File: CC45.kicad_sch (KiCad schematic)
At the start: 21 parts, among them J1 AVR-ISP-6, SW1 RESET, U1 ATmega32U4-AU, U2 PRTR5V0U2X, X1 XTAL

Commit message: add socket keep out zones
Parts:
- U1: footprint Package_QFP:TQFP-44_10x10mm_P0.8mm -> Package_QFP:TQFP-64_7x7mm_P0.4mm
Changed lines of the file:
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@@
   (junction (at 156.21 165.1) (diameter 0) (color 0 0 0 0))
   (no_connect (at 113.03 170.18))
-  (no_connect (at 64.77 72.39))
-  (no_connect (at 34.29 52.07))
+  (no_connect (at 113.03 154.94))
   (no_connect (at 64.77 36.83))
-  (no_connect (at 113.03 154.94))
   (no_connect (at 64.77 67.31))
   (no_connect (at 64.77 74.93))
+  (no_connect (at 34.29 52.07))
   (no_connect (at 64.77 69.85))
+  (no_connect (at 64.77 72.39))
   (wire (pts (xy 27.94 139.7) (xy 27.94 146.05))
     (stroke (width 0) (type solid) (color 0 0 0 0))
@@
     (property "Reference" "U1" (id 0) (at 39.37 120.65 0))
     (property "Value" "ATmega32U4-AU" (id 1) (at 36.83 123.19 0))
-    (property "Footprint" "Package_QFP:TQFP-44_10x10mm_P0.8mm" (id 2) (at 49.53 74.93 0)
+    (property "Footprint" "Package_QFP:TQFP-64_7x7mm_P0.4mm" (id 2) (at 49.53 74.93 0)
       (effects (font (size 1.27 1.27) italic) hide)
     )

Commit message: switch to 0805
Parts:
- C1, C2, C3, C4, C5, C6, C7, C8: footprint Capacitor_SMD:C_1206_3216Metric_Pad1.42x1.75mm_HandSolder -> Capacitor_SMD:C_0805_2012Metric
- R1, R2, R3, R4, R5, R6: footprint Resistor_SMD:R_1206_3216Metric_Pad1.42x1.75mm_HandSolder -> Resistor_SMD:R_0805_2012Metric
- U1: footprint Package_QFP:TQFP-64_7x7mm_P0.4mm -> libs:QFN44G-0.5-7X7MM
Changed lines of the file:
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@@
       (effects (font (size 1.27 1.27)) (justify right))
     )
-    (property "Footprint" "Resistor_SMD:R_1206_3216Metric_Pad1.42x1.75mm_HandSolder" (id 2) (at 40.64 175.26 0)
+    (property "Footprint" "Resistor_SMD:R_0805_2012Metric" (id 2) (at 40.64 175.26 0)
       (effects (font (size 1.27 1.27)) hide)
     )
@@
     (property "Reference" "R1" (id 0) (at 73.66 85.1916 90))
     (property "Value" "10k" (id 1) (at 73.66 87.503 90))
-    (property "Footprint" "Resistor_SMD:R_1206_3216Metric_Pad1.42x1.75mm_HandSolder" (id 2) (at 73.66 90.17 0)
+    (property "Footprint" "Resistor_SMD:R_0805_2012Metric" (id 2) (at 73.66 90.17 0)
       (effects (font (size 1.27 1.27)) hide)
     )
@@
     (property "Reference" "R5" (id 0) (at 116.84 175.26 90))
     (property "Value" "5.1k" (id 1) (at 119.38 175.26 90))
-    (property "Footprint" "Resistor_SMD:R_1206_3216Metric_Pad1.42x1.75mm_HandSolder" (id 2) (at 121.92 175.26 0)
+    (property "Footprint" "Resistor_SMD:R_0805_2012Metric" (id 2) (at 121.92 175.26 0)
       (effects (font (size 1.27 1.27)) hide)
     )
@@
     (property "Reference" "R6" (id 0) (at 125.73 175.26 90))
     (property "Value" "5.1k" (id 1) (at 128.27 175.26 90))
-    (property "Footprint" "Resistor_SMD:R_1206_3216Metric_Pad1.42x1.75mm_HandSolder" (id 2) (at 130.81 175.26 0)
+    (property "Footprint" "Resistor_SMD:R_0805_2012Metric" (id 2) (at 130.81 175.26 0)
       (effects (font (size 1.27 1.27)) hide)
     )
@@
     (property "Reference" "R2" (id 0) (at 162.56 160.02 90))
     (property "Value" "22" (id 1) (at 162.56 162.56 90))
-    (property "Footprint" "Resistor_SMD:R_1206_3216Metric_Pad1.42x1.75mm_HandSolder" (id 2) (at 162.56 165.1 0)
+    (property "Footprint" "Resistor_SMD:R_0805_2012Metric" (id 2) (at 162.56 165.1 0)
       (effects (font (size 1.27 1.27)) hide)
     )
@@
     (property "Reference" "R3" (id 0) (at 162.56 172.72 90))
     (property "Value" "22" (id 1) (at 162.56 170.18 90))
-    (property "Footprint" "Resistor_SMD:R_1206_3216Metric_Pad1.42x1.75mm_HandSolder" (id 2) (at 162.56 167.64 0)
+    (property "Footprint" "Resistor_SMD:R_0805_2012Metric" (id 2) (at 162.56 167.64 0)
       (effects (font (size 1.27 1.27)) hide)
     )
@@
       (effects (font (size 1.27 1.27)) (justify left))
     )
-    (property "Footprint" "Capacitor_SMD:C_1206_3216Metric_Pad1.42x1.75mm_HandSolder" (id 2) (at 27.94 151.13 0)
+    (property "Footprint" "Capacitor_SMD:C_0805_2012Metric" (id 2) (at 27.94 151.13 0)
       (effects (font (size 1.27 1.27)) hide)
     )
@@
       (effects (font (size 1.27 1.27)) (justify left))
     )
-    (property "Footprint" "Capacitor_SMD:C_1206_3216Metric_Pad1.42x1.75mm_HandSolder" (id 2) (at 30.48 74.93 0)
+    (property "Footprint" "Capacitor_SMD:C_0805_2012Metric" (id 2) (at 30.48 74.93 0)
       (effects (font (size 1.27 1.27)) hide)
     )
@@
       (effects (font (size 1.27 1.27)) (justify left))
     )
-    (property "Footprint" "Capacitor_SMD:C_1206_3216Metric_Pad1.42x1.75mm_HandSolder" (id 2) (at 43.18 151.13 0)
+    (property "Footprint" "Capacitor_SMD:C_0805_2012Metric" (id 2) (at 43.18 151.13 0)
       (effects (font (size 1.27 1.27)) hide)
     )
@@
       (effects (font (size 1.27 1.27)) (justify left))
     )
-    (property "Footprint" "Capacitor_SMD:C_1206_3216Metric_Pad1.42x1.75mm_HandSolder" (id 2) (at 52.07 135.255 0)
+    (property "Footprint" "Capacitor_SMD:C_0805_2012Metric" (id 2) (at 52.07 135.255 0)
       (effects (font (size 1.27 1.27)) hide)
     )
@@
       (effects (font (size 1.27 1.27)) (justify left))
     )
-    (property "Footprint" "Capacitor_SMD:C_1206_3216Metric_Pad1.42x1.75mm_HandSolder" (id 2) (at 59.69 135.255 0)
+    (property "Footprint" "Capacitor_SMD:C_0805_2012Metric" (id 2) (at 59.69 135.255 0)
       (effects (font (size 1.27 1.27)) hide)
     )
@@
       (effects (font (size 1.27 1.27)) (justify left))
     )
-    (property "Footprint" "Capacitor_SMD:C_1206_3216Metric_Pad1.42x1.75mm_HandSolder" (id 2) (at 68.58 135.255 0)
+    (property "Footprint" "Capacitor_SMD:C_0805_2012Metric" (id 2) (at 68.58 135.255 0)
       (effects (font (size 1.27 1.27)) hide)
     )
@@
       (effects (font (size 1.27 1.27)) (justify left))
     )
-    (property "Footprint" "Capacitor_SMD:C_1206_3216Metric_Pad1.42x1.75mm_HandSolder" (id 2) (at 78.74 135.255 0)
+    (property "Footprint" "Capacitor_SMD:C_0805_2012Metric" (id 2) (at 78.74 135.255 0)
       (effects (font (size 1.27 1.27)) hide)
     )
@@
       (effects (font (size 1.27 1.27)) (justify left))
     )
-    (property "Footprint" "Capacitor_SMD:C_1206_3216Metric_Pad1.42x1.75mm_HandSolder" (id 2) (at 87.63 135.255 0)
+    (property "Footprint" "Capacitor_SMD:C_0805_2012Metric" (id 2) (at 87.63 135.255 0)
       (effects (font (size 1.27 1.27)) hide)
     )
@@
     (property "Reference" "U1" (id 0) (at 39.37 120.65 0))
     (property "Value" "ATmega32U4-AU" (id 1) (at 36.83 123.19 0))
-    (property "Footprint" "Package_QFP:TQFP-64_7x7mm_P0.4mm" (id 2) (at 49.53 74.93 0)
+    (property "Footprint" "libs:QFN44G-0.5-7X7MM" (id 2) (at 49.53 74.93 0)
       (effects (font (size 1.27 1.27) italic) hide)
     )

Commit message: switch to 0603
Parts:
- C1, C2, C3, C4, C5, C6, C7, C8: footprint Capacitor_SMD:C_0805_2012Metric -> Capacitor_SMD:C_0603_1608Metric
- R1, R2, R3, R4, R5, R6: footprint Resistor_SMD:R_0805_2012Metric -> Resistor_SMD:R_0603_1608Metric
- X1: footprint Crystal:Crystal_SMD_3225-4Pin_3.2x2.5mm_HandSoldering -> Crystal:Crystal_SMD_2016-4Pin_2.0x1.6mm
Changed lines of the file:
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@@
       (effects (font (size 1.27 1.27)) (justify right))
     )
-    (property "Footprint" "Resistor_SMD:R_0805_2012Metric" (id 2) (at 40.64 175.26 0)
+    (property "Footprint" "Resistor_SMD:R_0603_1608Metric" (id 2) (at 40.64 175.26 0)
       (effects (font (size 1.27 1.27)) hide)
     )
@@
     (property "Reference" "R1" (id 0) (at 73.66 85.1916 90))
     (property "Value" "10k" (id 1) (at 73.66 87.503 90))
-    (property "Footprint" "Resistor_SMD:R_0805_2012Metric" (id 2) (at 73.66 90.17 0)
+    (property "Footprint" "Resistor_SMD:R_0603_1608Metric" (id 2) (at 73.66 90.17 0)
       (effects (font (size 1.27 1.27)) hide)
     )
@@
     (property "Reference" "R5" (id 0) (at 116.84 175.26 90))
     (property "Value" "5.1k" (id 1) (at 119.38 175.26 90))
-    (property "Footprint" "Resistor_SMD:R_0805_2012Metric" (id 2) (at 121.92 175.26 0)
+    (property "Footprint" "Resistor_SMD:R_0603_1608Metric" (id 2) (at 121.92 175.26 0)
       (effects (font (size 1.27 1.27)) hide)
     )
@@
     (property "Reference" "R6" (id 0) (at 125.73 175.26 90))
     (property "Value" "5.1k" (id 1) (at 128.27 175.26 90))
-    (property "Footprint" "Resistor_SMD:R_0805_2012Metric" (id 2) (at 130.81 175.26 0)
+    (property "Footprint" "Resistor_SMD:R_0603_1608Metric" (id 2) (at 130.81 175.26 0)
       (effects (font (size 1.27 1.27)) hide)
     )
@@
     (property "Reference" "R2" (id 0) (at 162.56 160.02 90))
     (property "Value" "22" (id 1) (at 162.56 162.56 90))
-    (property "Footprint" "Resistor_SMD:R_0805_2012Metric" (id 2) (at 162.56 165.1 0)
+    (property "Footprint" "Resistor_SMD:R_0603_1608Metric" (id 2) (at 162.56 165.1 0)
       (effects (font (size 1.27 1.27)) hide)
     )
@@
     (property "Reference" "R3" (id 0) (at 162.56 172.72 90))
     (property "Value" "22" (id 1) (at 162.56 170.18 90))
-    (property "Footprint" "Resistor_SMD:R_0805_2012Metric" (id 2) (at 162.56 167.64 0)
+    (property "Footprint" "Resistor_SMD:R_0603_1608Metric" (id 2) (at 162.56 167.64 0)
       (effects (font (size 1.27 1.27)) hide)
     )
@@
       (effects (font (size 1.27 1.27)) (justify left))
     )
-    (property "Footprint" "Capacitor_SMD:C_0805_2012Metric" (id 2) (at 27.94 151.13 0)
+    (property "Footprint" "Capacitor_SMD:C_0603_1608Metric" (id 2) (at 27.94 151.13 0)
       (effects (font (size 1.27 1.27)) hide)
     )
@@
       (effects (font (size 1.27 1.27)) (justify left))
     )
-    (property "Footprint" "Capacitor_SMD:C_0805_2012Metric" (id 2) (at 30.48 74.93 0)
+    (property "Footprint" "Capacitor_SMD:C_0603_1608Metric" (id 2) (at 30.48 74.93 0)
       (effects (font (size 1.27 1.27)) hide)
     )
@@
       (effects (font (size 1.27 1.27)) (justify left))
     )
-    (property "Footprint" "Capacitor_SMD:C_0805_2012Metric" (id 2) (at 43.18 151.13 0)
+    (property "Footprint" "Capacitor_SMD:C_0603_1608Metric" (id 2) (at 43.18 151.13 0)
       (effects (font (size 1.27 1.27)) hide)
     )
@@
       (effects (font (size 1.27 1.27)) (justify left))
     )
-    (property "Footprint" "Capacitor_SMD:C_0805_2012Metric" (id 2) (at 52.07 135.255 0)
+    (property "Footprint" "Capacitor_SMD:C_0603_1608Metric" (id 2) (at 52.07 135.255 0)
       (effects (font (size 1.27 1.27)) hide)
     )
@@
       (effects (font (size 1.27 1.27)) (justify left))
     )
-    (property "Footprint" "Capacitor_SMD:C_0805_2012Metric" (id 2) (at 59.69 135.255 0)
+    (property "Footprint" "Capacitor_SMD:C_0603_1608Metric" (id 2) (at 59.69 135.255 0)
       (effects (font (size 1.27 1.27)) hide)
     )
@@
       (effects (font (size 1.27 1.27)) (justify left))
     )
-    (property "Footprint" "Capacitor_SMD:C_0805_2012Metric" (id 2) (at 68.58 135.255 0)
+    (property "Footprint" "Capacitor_SMD:C_0603_1608Metric" (id 2) (at 68.58 135.255 0)
       (effects (font (size 1.27 1.27)) hide)
     )
@@
       (effects (font (size 1.27 1.27)) (justify left))
     )
-    (property "Footprint" "Capacitor_SMD:C_0805_2012Metric" (id 2) (at 78.74 135.255 0)
+    (property "Footprint" "Capacitor_SMD:C_0603_1608Metric" (id 2) (at 78.74 135.255 0)
       (effects (font (size 1.27 1.27)) hide)
     )
@@
       (effects (font (size 1.27 1.27)) (justify left))
     )
-    (property "Footprint" "Capacitor_SMD:C_0805_2012Metric" (id 2) (at 87.63 135.255 0)
+    (property "Footprint" "Capacitor_SMD:C_0603_1608Metric" (id 2) (at 87.63 135.255 0)
       (effects (font (size 1.27 1.27)) hide)
     )
@@
       (effects (font (size 1.27 1.27)) (justify left))
     )
-    (property "Footprint" "Crystal:Crystal_SMD_3225-4Pin_3.2x2.5mm_HandSoldering" (id 2) (at 35.56 146.05 0)
-      (effects (font (size 1.27 1.27)) hide)
-    )
+    (property "Footprint" "Crystal:Crystal_SMD_2016-4Pin_2.0x1.6mm" (id 2) (at 35.56 146.05 0)
+      (effects (font (size 1.27 1.27)) hide)
+    )

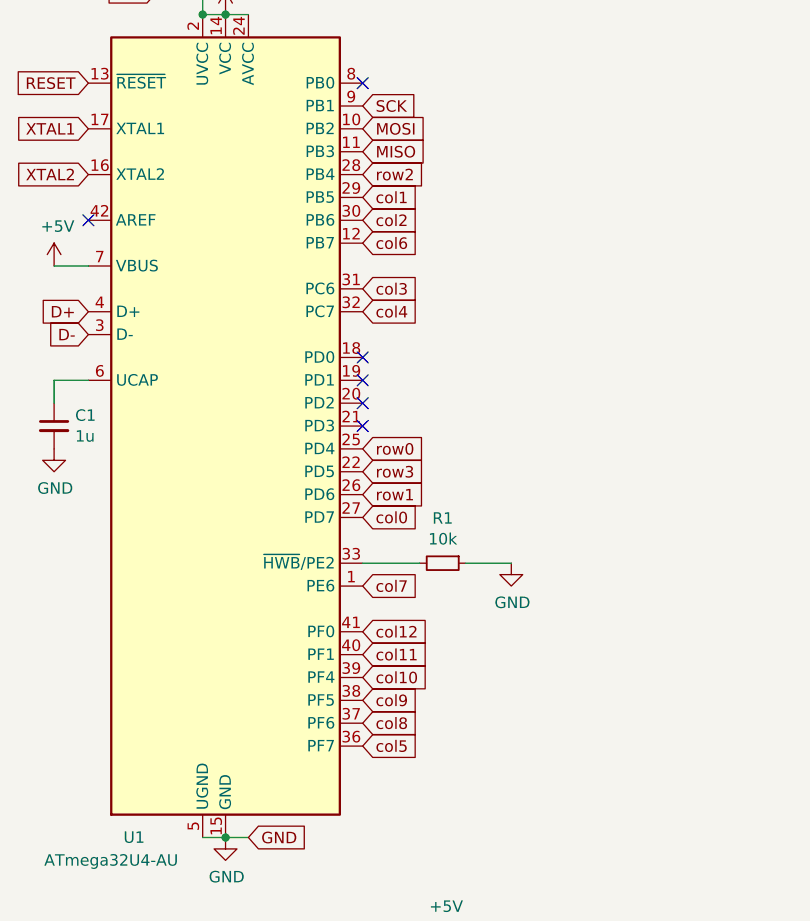
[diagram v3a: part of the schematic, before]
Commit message: routing lol
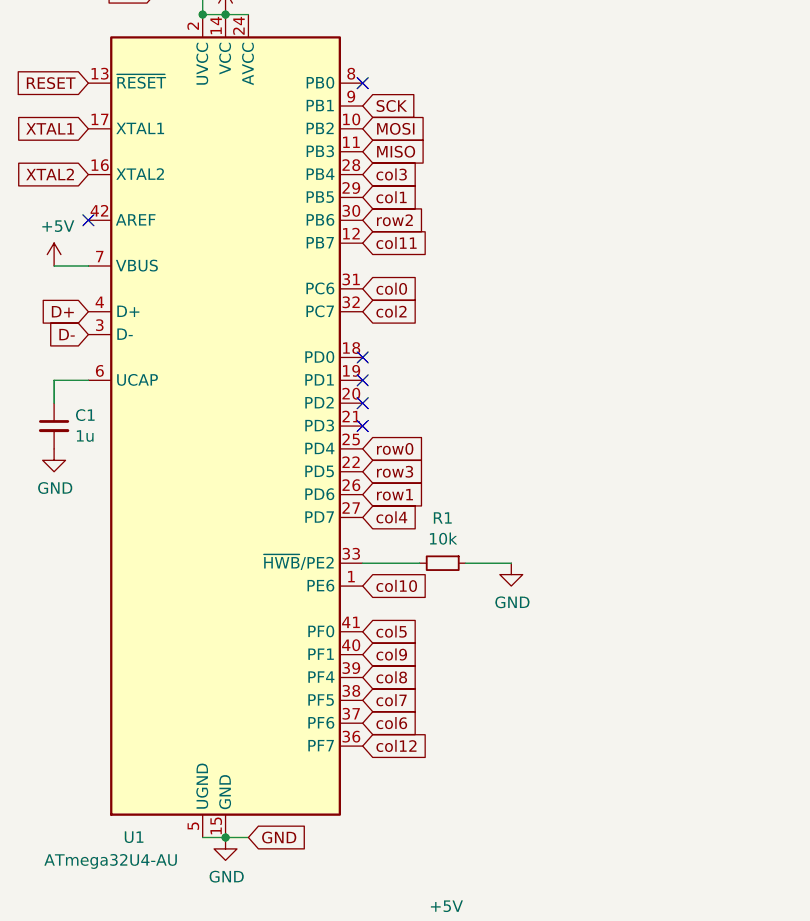
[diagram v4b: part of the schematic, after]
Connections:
- net col0: now also U1.31 (PC6); no longer U1.27 (PD7)
- net col10: now also U1.1 (PE6); no longer U1.39 (PF4)
- net col11: now also U1.12 (PB7); no longer U1.40 (PF1)
- net col12: now also U1.36 (PF7); no longer U1.41 (PF0)
- net col2: now also U1.32 (PC7); no longer U1.30 (PB6)
- net col3: now also U1.28 (PB4); no longer U1.31 (PC6)
- net col4: now also U1.27 (PD7); no longer U1.32 (PC7)
- net col5: now also U1.41 (PF0); no longer U1.36 (PF7)
- net col6: now also U1.37 (PF6); no longer U1.12 (PB7)
- net col7: now also U1.38 (PF5); no longer U1.1 (PE6)
- net col8: now also U1.39 (PF4); no longer U1.37 (PF6)
- net col9: now also U1.40 (PF1); no longer U1.38 (PF5)
- net row2: now also U1.30 (PB6); no longer U1.28 (PB4)
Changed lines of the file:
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@@
     (effects (font (size 1.27 1.27)) (justify left))
   )
-  (global_label "row2" (shape input) (at 64.77 46.99 0)
+  (global_label "col3" (shape input) (at 64.77 46.99 0)
     (effects (font (size 1.27 1.27)) (justify left))
   )
@@
     (effects (font (size 1.27 1.27)) (justify left))
   )
-  (global_label "col2" (shape input) (at 64.77 52.07 0)
+  (global_label "row2" (shape input) (at 64.77 52.07 0)
     (effects (font (size 1.27 1.27)) (justify left))
   )
-  (global_label "col6" (shape input) (at 64.77 54.61 0)
+  (global_label "col11" (shape input) (at 64.77 54.61 0)
     (effects (font (size 1.27 1.27)) (justify left))
   )
-  (global_label "col3" (shape input) (at 64.77 59.69 0)
+  (global_label "col0" (shape input) (at 64.77 59.69 0)
     (effects (font (size 1.27 1.27)) (justify left))
   )
-  (global_label "col4" (shape input) (at 64.77 62.23 0)
+  (global_label "col2" (shape input) (at 64.77 62.23 0)
     (effects (font (size 1.27 1.27)) (justify left))
   )
@@
     (effects (font (size 1.27 1.27)) (justify left))
   )
-  (global_label "col0" (shape input) (at 64.77 85.09 0)
+  (global_label "col4" (shape input) (at 64.77 85.09 0)
     (effects (font (size 1.27 1.27)) (justify left))
   )
-  (global_label "col7" (shape input) (at 64.77 92.71 0)
+  (global_label "col10" (shape input) (at 64.77 92.71 0)
     (effects (font (size 1.27 1.27)) (justify left))
   )
-  (global_label "col12" (shape input) (at 64.77 97.79 0)
+  (global_label "col5" (shape input) (at 64.77 97.79 0)
     (effects (font (size 1.27 1.27)) (justify left))
   )
-  (global_label "col11" (shape input) (at 64.77 100.33 0)
+  (global_label "col9" (shape input) (at 64.77 100.33 0)
     (effects (font (size 1.27 1.27)) (justify left))
   )
-  (global_label "col10" (shape input) (at 64.77 102.87 0)
+  (global_label "col8" (shape input) (at 64.77 102.87 0)
     (effects (font (size 1.27 1.27)) (justify left))
   )
-  (global_label "col9" (shape input) (at 64.77 105.41 0)
+  (global_label "col7" (shape input) (at 64.77 105.41 0)
     (effects (font (size 1.27 1.27)) (justify left))
   )
-  (global_label "col8" (shape input) (at 64.77 107.95 0)
+  (global_label "col6" (shape input) (at 64.77 107.95 0)
     (effects (font (size 1.27 1.27)) (justify left))
   )
-  (global_label "col5" (shape input) (at 64.77 110.49 0)
+  (global_label "col12" (shape input) (at 64.77 110.49 0)
     (effects (font (size 1.27 1.27)) (justify left))
   )
